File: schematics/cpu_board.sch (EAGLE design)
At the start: 7 parts, among them IC2 7404N, IC3 74LS245N, IC4 74367N, IC5 74367N, IC6 74367N

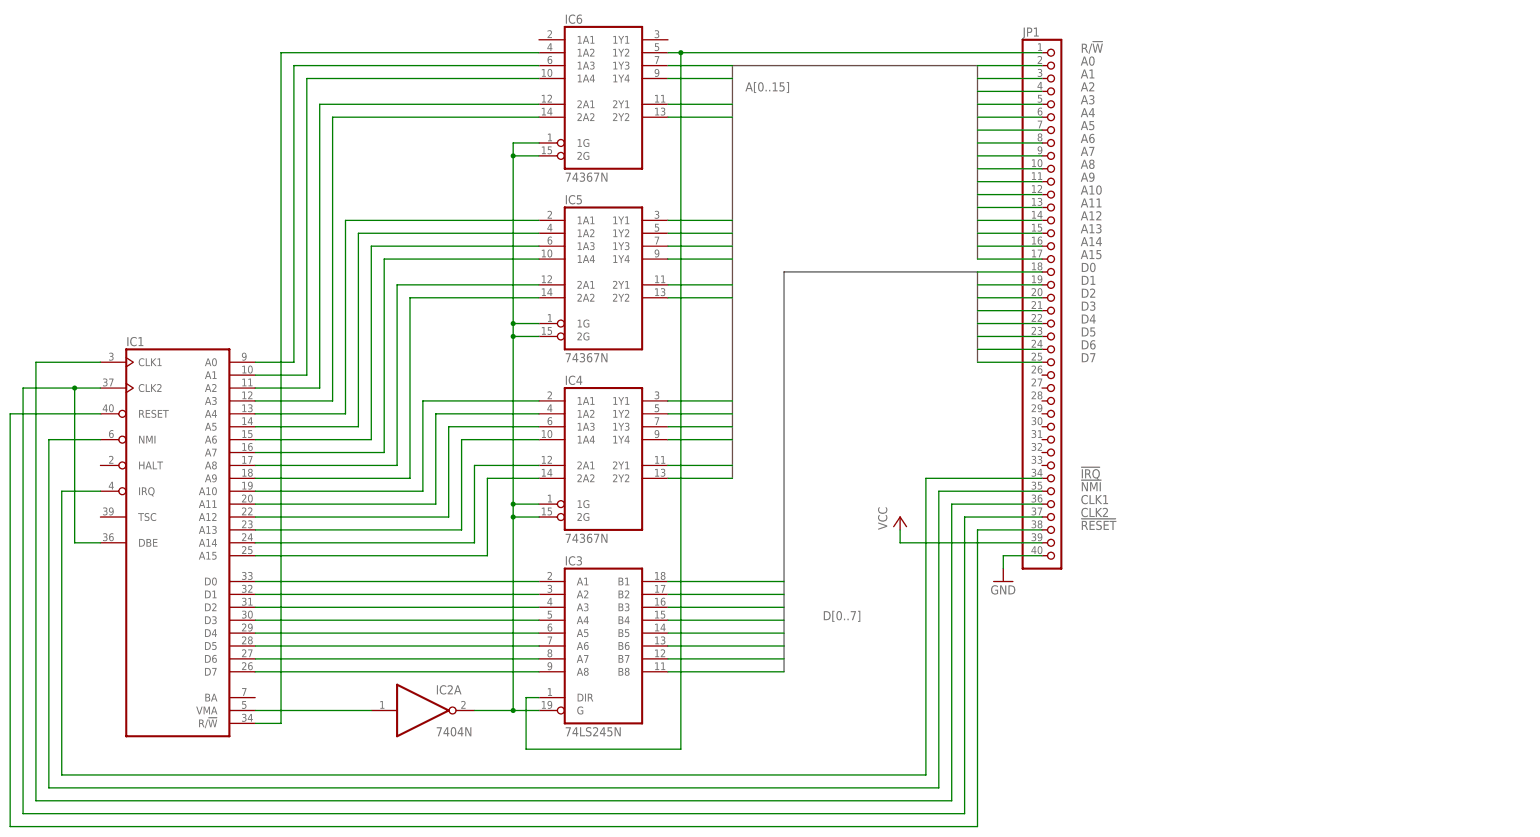
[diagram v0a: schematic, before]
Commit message: Memorias
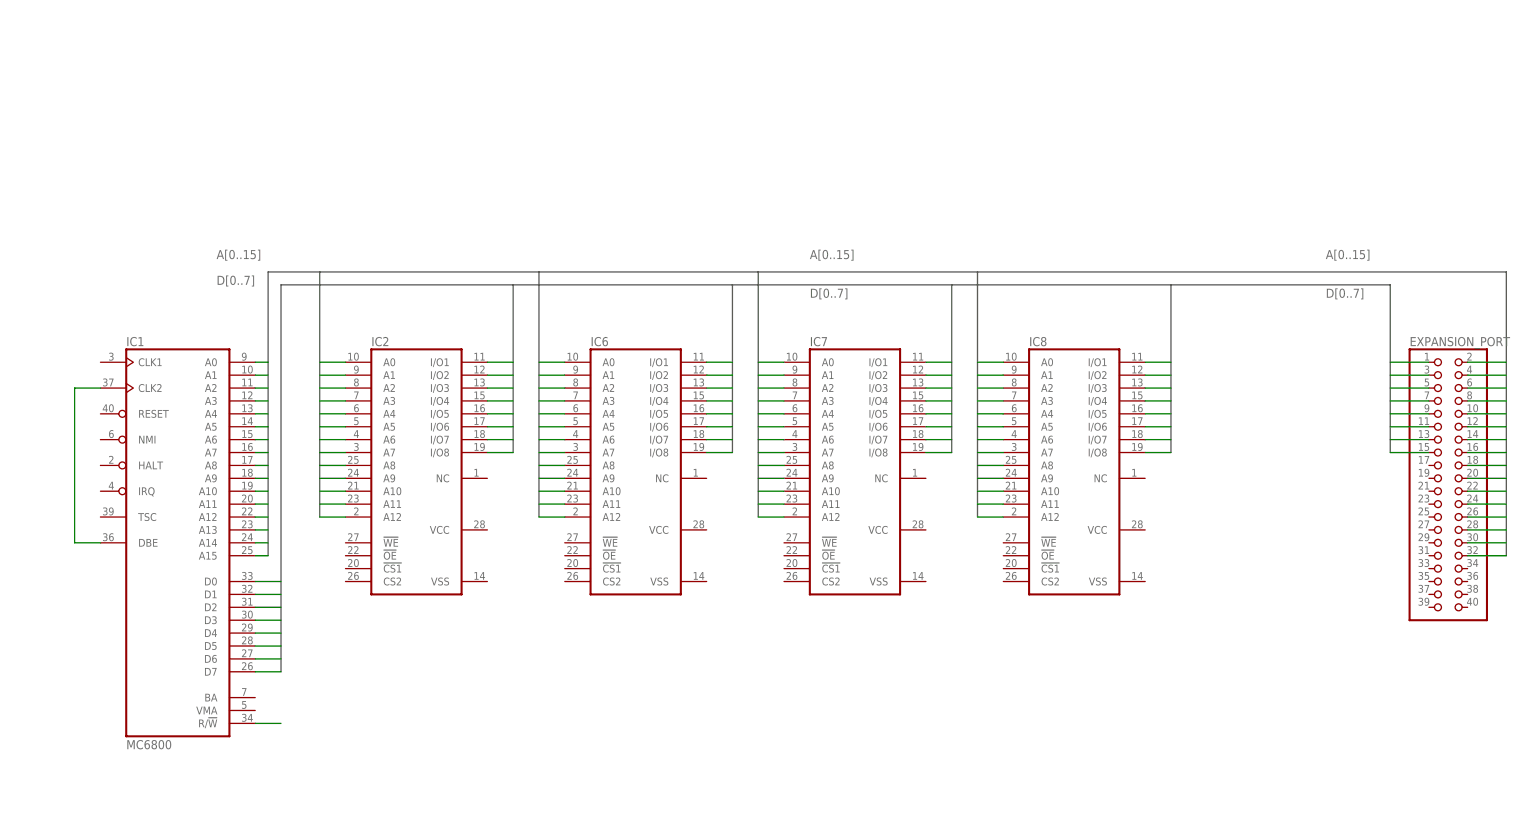
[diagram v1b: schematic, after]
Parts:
- removed IC3: 74LS245N, 74xx-us:74LS245N
- removed IC4, IC5: 74367N, 74xx-us:74367N
- removed JP1: (no value), pinhead:PINHD-1X40
- added EXPANSION_PORT: (no value), pinhead:PINHD-2X20
- added IC7, IC8: (no value), memory-hitachi:6264A
- IC1: value (none) -> MC6800
- IC2: value 7404N -> (none); device 74xx-us:7404N -> memory-hitachi:6264A
- IC6: value 74367N -> (none); device 74xx-us:74367N -> memory-hitachi:6264A
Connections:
- removed net !IRQ: IC1A.IRQ, JP1.34
- removed net !NMI: IC1A.NMI, JP1.35
- removed net !RESET: IC1A.RESET, JP1.38
- removed net CLK1: IC1A.CLK1, JP1.36
- removed net CLK2: IC1A.CLK2, IC1A.DBE, JP1.37
- removed net GND: JP1.40
- removed net N$1: IC1A.D0, IC3A.A1
- removed net N$10: IC1A.VMA, IC2A.I
- removed net N$11: IC2A.O, IC3A.G, IC4A.1G, IC4A.2G, IC5A.1G, IC5A.2G, IC6A.1G, IC6A.2G
- removed net N$12: IC1A.A14, IC4A.2A1
- removed net N$13: IC1A.A13, IC4A.1A4
- removed net N$14: IC1A.A12, IC4A.1A3
- removed net N$15: IC1A.A11, IC4A.1A2
- removed net N$16: IC1A.A10, IC4A.1A1
- removed net N$17: IC1A.A9, IC5A.2A2
- removed net N$18: IC1A.A8, IC5A.2A1
- removed net N$19: IC1A.A7, IC5A.1A4
- removed net N$20: IC1A.A6, IC5A.1A3
- removed net N$21: IC1A.A5, IC5A.1A2
- removed net N$22: IC1A.A4, IC5A.1A1
- removed net N$23: IC1A.A3, IC6A.2A2
- removed net N$24: IC1A.A2, IC6A.2A1
- removed net N$25: IC1A.A1, IC6A.1A4
- removed net N$26: IC1A.A0, IC6A.1A3
- removed net N$27: IC1A.R/!W, IC6A.1A2
- removed net N$3: IC1A.D2, IC3A.A3
- removed net N$4: IC1A.D3, IC3A.A4
- removed net N$5: IC1A.D4, IC3A.A5
- removed net N$6: IC1A.D5, IC3A.A6
- removed net N$7: IC1A.D6, IC3A.A7
- removed net N$9: IC1A.A15, IC4A.2A2
- removed net R/!W: IC3A.DIR, IC6A.1Y2, JP1.1
- removed net VCC: JP1.39
- net A0: now also EXPANSION_PORT.2, IC1A.A0, IC2.A0, IC6.A0, IC7.A0, IC8.A0; no longer IC6A.1Y3, JP1.2
- net A1: now also EXPANSION_PORT.4, IC1A.A1, IC2.A1, IC6.A1, IC7.A1, IC8.A1; no longer IC6A.1Y4, JP1.3
- net A10: now also EXPANSION_PORT.22, IC1A.A10, IC2.A10, IC6.A10, IC7.A10, IC8.A10; no longer IC4A.1Y1, JP1.12
- net A11: now also EXPANSION_PORT.24, IC1A.A11, IC2.A11, IC6.A11, IC7.A11, IC8.A11; no longer IC4A.1Y2, JP1.13
- net A12: now also EXPANSION_PORT.26, IC1A.A12, IC2.A12, IC6.A12, IC7.A12, IC8.A12; no longer IC4A.1Y3, JP1.14
- net A13: now also EXPANSION_PORT.28, IC1A.A13; no longer IC4A.1Y4, JP1.15
- net A14: now also EXPANSION_PORT.30, IC1A.A14; no longer IC4A.2Y1, JP1.16
- net A15: now also EXPANSION_PORT.32, IC1A.A15; no longer IC4A.2Y2, JP1.17
- net A2: now also EXPANSION_PORT.6, IC1A.A2, IC2.A2, IC6.A2, IC7.A2, IC8.A2; no longer IC6A.2Y1, JP1.4
- net A3: now also EXPANSION_PORT.8, IC1A.A3, IC2.A3, IC6.A3, IC7.A3, IC8.A3; no longer IC6A.2Y2, JP1.5
- net A4: now also EXPANSION_PORT.10, IC1A.A4, IC2.A4, IC6.A4, IC7.A4, IC8.A4; no longer IC5A.1Y1, JP1.6
- net A5: now also EXPANSION_PORT.12, IC1A.A5, IC2.A5, IC6.A5, IC7.A5, IC8.A5; no longer IC5A.1Y2, JP1.7
- net A6: now also EXPANSION_PORT.14, IC1A.A6, IC2.A6, IC6.A6, IC7.A6, IC7.A7, IC8.A6; no longer IC5A.1Y3, JP1.8
- net A7: now also EXPANSION_PORT.16, IC1A.A7, IC2.A7, IC6.A7, IC8.A7; no longer IC5A.1Y4, JP1.9
- net A8: now also EXPANSION_PORT.18, IC1A.A8, IC2.A8, IC6.A8, IC7.A8, IC8.A8; no longer IC5A.2Y1, JP1.10
- net A9: now also EXPANSION_PORT.20, IC1A.A9, IC2.A9, IC6.A9, IC7.A9, IC8.A9; no longer IC5A.2Y2, JP1.11
- net D0: now also EXPANSION_PORT.1, IC1A.D0, IC2.I/O1, IC6.I/O1, IC7.I/O1, IC8.I/O1; no longer IC3A.B1, JP1.18
- net D1: now also EXPANSION_PORT.3, IC1A.D1, IC2.I/O2, IC6.I/O2, IC7.I/O2, IC8.I/O2; no longer IC3A.B2, JP1.19
- net D2: now also EXPANSION_PORT.5, IC1A.D2, IC2.I/O3, IC6.I/O3, IC7.I/O3, IC8.I/O3; no longer IC3A.B3, JP1.20
- net D3: now also EXPANSION_PORT.7, IC1A.D3, IC2.I/O4, IC6.I/O4, IC7.I/O4, IC8.I/O4; no longer IC3A.B4, JP1.21
- net D4: now also EXPANSION_PORT.9, IC1A.D4, IC2.I/O5, IC6.I/O5, IC7.I/O5, IC8.I/O5; no longer IC3A.B5, JP1.22
- net D5: now also EXPANSION_PORT.11, IC1A.D5, IC2.I/O6, IC6.I/O6, IC7.I/O6, IC8.I/O6; no longer IC3A.B6, JP1.23
- net D6: now also EXPANSION_PORT.13, IC1A.D6, IC2.I/O7, IC6.I/O7, IC7.I/O7, IC8.I/O7; no longer IC3A.B7, JP1.24
- net D7: now also EXPANSION_PORT.15, IC1A.D7, IC2.I/O8, IC6.I/O8, IC7.I/O8, IC8.I/O8; no longer IC3A.B8, JP1.25
- net N$2: now also IC1A.CLK2, IC1A.DBE; no longer IC1A.D1, IC3A.A2
- net N$8: now also IC1A.R/!W; no longer IC1A.D7, IC3A.A8
